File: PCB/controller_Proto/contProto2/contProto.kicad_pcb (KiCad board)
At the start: 2 copper layers, 130.9 x 105.1 mm, 84 parts, among them J1 JST_1mm_4, J10 JST_1mm_3, J11 JST_1mm_3, J12 Conn_01x03_Socket, J13 Conn_01x02_Socket, J14 Conn_01x02_Socket, J15 Conn_01x04, J16 Conn_01x04, J17 Conn_01x10_Pin, J18 JST_1mm_3, J19 Conn_01x08_Socket, J2 Conn_01x04, J20 JST_1mm_4, J22 JST_1mm_4, J23 Conn_01x03_Socket, J24 Conn_01x03_Socket, J25 Conn_01x03_Socket, J26 Conn_01x03_Socket, J27 Conn_01x03_Socket, J28 Conn_01x12_Socket, J29 Conn_01x12_Socket, J3 Conn_01x10_Pin, J30 Conn_01x12_Socket, J31 Conn_01x12_Socket, J32 Conn_01x03_Socket, J33 Conn_01x03_Socket, J36 Conn_01x05, J37 Conn_01x05, J4 JST_1mm_3, J5 Conn_01x02_Socket, J6 JST_1mm_3, J7 Conn_01x02_Socket, J8 JST_1mm_4, J9 Conn_01x04, SW1 SMD_12x12mm_h8.5mm, SW10 SMD_12x12mm_h8.5mm, SW11 SMD_12x12mm_h8.5mm, SW12 SMD_12x12mm_h8.5mm, SW13 SMD_12x12mm_h8.5mm, SW14 SMD_12x12mm_h8.5mm, SW15 SMD_12x12mm_h8.5mm, SW16 SMD_12x12mm_h8.5mm, SW17 SMD_12x12mm_h8.5mm, SW18 SMD_12x12mm_h8.5mm, SW19 SMD_12x12mm_h8.5mm, SW2 SMD_12x12mm_h8.5mm, SW20 SMD_12x12mm_h8.5mm, SW3 SMD_12x12mm_h8.5mm, SW4 SMD_12x12mm_h8.5mm, SW5 SMD_12x12mm_h8.5mm, SW6 SMD_12x12mm_h8.5mm, SW7 SMD_12x12mm_h8.5mm, SW8 SMD_12x12mm_h8.5mm, SW9 SMD_12x12mm_h8.5mm, U1 ProMicroC, U2 ProMicroC, U3 DRV5033FAxLPG, U4 DRV5033FAxLPG

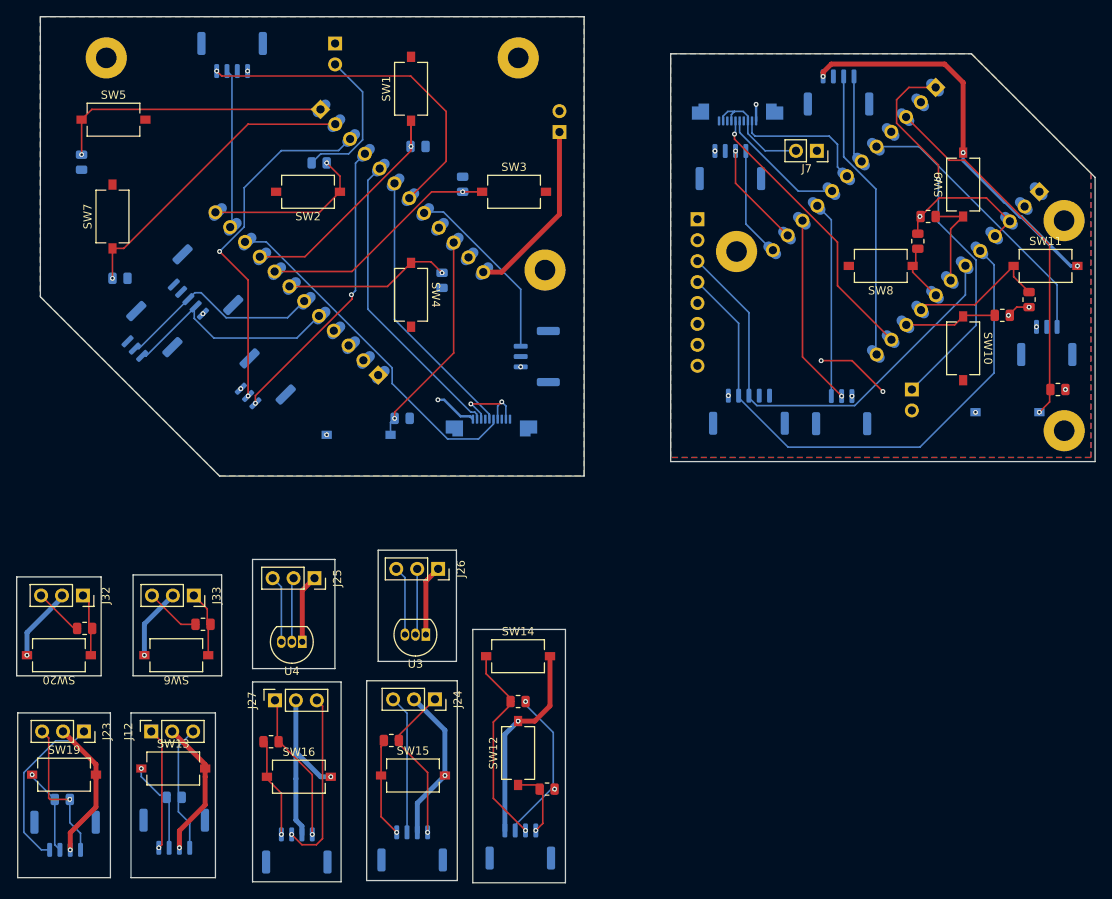
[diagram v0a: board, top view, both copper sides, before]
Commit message: final pcb
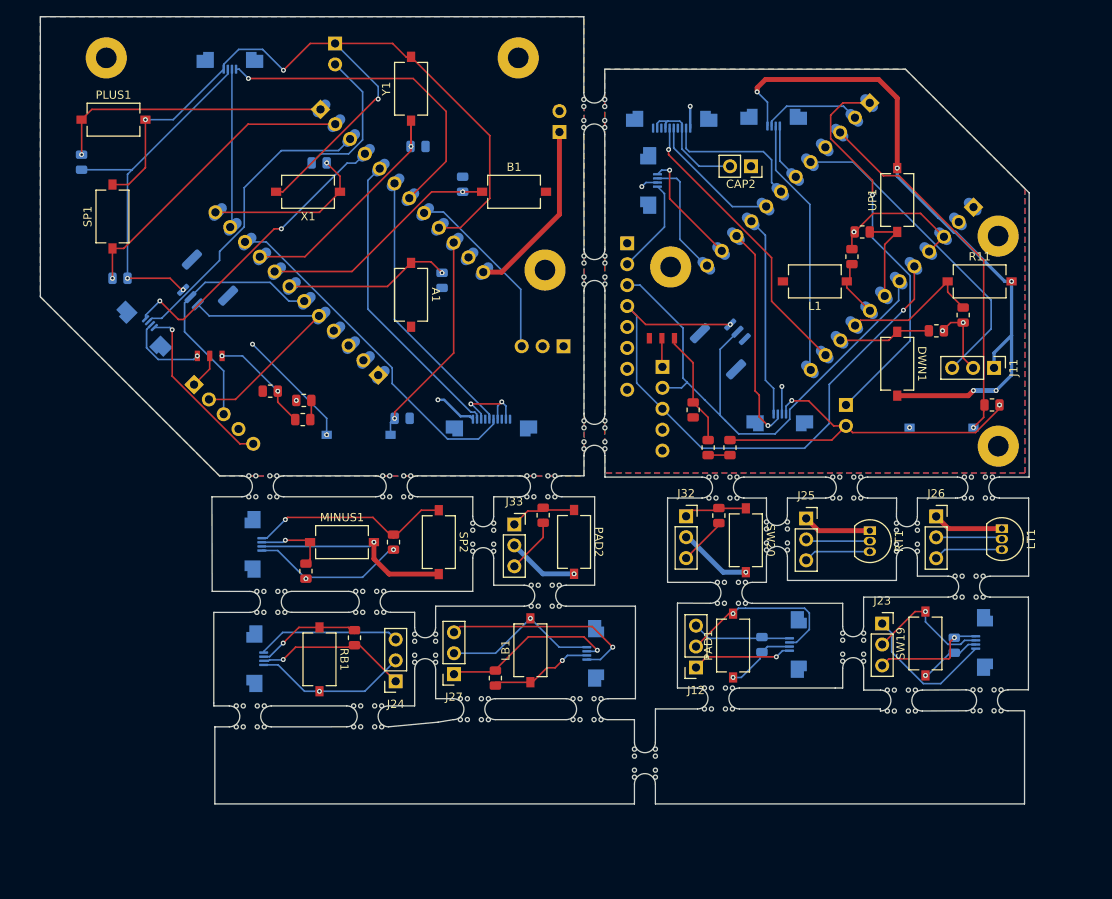
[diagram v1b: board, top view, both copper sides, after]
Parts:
- removed J1, J20, J22, J8: JST_1mm_4, Connector_JST:JST_GH_BM04B-GHS-TBT_1x04-1MP_P1.25mm_Vertical
- removed J15, J16, J2: Conn_01x04, Connector_JST:JST_GH_BM04B-GHS-TBT_1x04-1MP_P1.25mm_Vertical
- removed J36: Conn_01x05, Connector_JST:JST_GH_BM05B-GHS-TBT_1x05-1MP_P1.25mm_Vertical
- removed J6: JST_1mm_3, Connector_JST:JST_GH_BM03B-GHS-TBT_1x03-1MP_P1.25mm_Vertical
- added JP1: ~, PCM_SparkFun-Jumper:Jumper_3_NO, F.Cu at (99.9, 61.5)
- added JP2: ~, PCM_SparkFun-Jumper:Jumper_3_NO, F.Cu at (45.0, 63.7)
- added L_SHOUL1: Conn_01x04, Connector_FFC-FPC:Amphenol_F32Q-1A7x1-11004_1x04-1MP_P0.5mm_Horizontal, B.Cu at (93.7, 99.8)
- added PAD3: Conn_01x04, Connector_FFC-FPC:Amphenol_F32Q-1A7x1-11004_1x04-1MP_P0.5mm_Horizontal, B.Cu at (35.8, 61.8)
- added PAD4: Conn_01x04, Connector_FFC-FPC:Amphenol_F32Q-1A7x1-11004_1x04-1MP_P0.5mm_Horizontal, B.Cu at (114.2, 73.6)
- added PAD_B1: Conn_01x04, Connector_FFC-FPC:Amphenol_F32Q-1A7x1-11004_1x04-1MP_P0.5mm_Horizontal, B.Cu at (118.3, 98.7)
- added PAD_B2: Conn_01x04, Connector_FFC-FPC:Amphenol_F32Q-1A7x1-11004_1x04-1MP_P0.5mm_Horizontal, B.Cu at (140.9, 98.5)
- added R12: 1k, PCM_SparkFun-Resistor:R_0805_2012Metric, F.Cu at (52.4, 68.0)
- added R23: 1k, PCM_SparkFun-Resistor:R_0805_2012Metric, F.Cu at (56.4, 71.4)
- added R24: 1k, PCM_SparkFun-Resistor:R_0805_2012Metric, F.Cu at (103.7, 70.2)
- added R25: 1k, PCM_SparkFun-Resistor:R_0805_2012Metric, F.Cu at (105.5, 74.8)
- added R26: 1k, PCM_SparkFun-Resistor:R_0805_2012Metric, F.Cu at (56.5, 69.1)
- added R27: 1k, PCM_SparkFun-Resistor:R_0805_2012Metric, F.Cu at (108.2, 74.8)
- added REF**: MouseBite-Slot_2.54x2.54mm_on-edge_D0.5mm_P0.85mm_4h_Trace, Panelization:MouseBite-Slot_2.54x2.54mm_on-edge_D0.5mm_P0.85mm_4h_Trace, F.Cu at (52.5, 92.3)
- added REF**: MouseBite-Slot_2.54x2.54mm_on-edge_D0.5mm_P0.85mm_4h_Trace, Panelization:MouseBite-Slot_2.54x2.54mm_on-edge_D0.5mm_P0.85mm_4h_Trace, F.Cu at (64.5, 92.2)
- added REF**: MouseBite-Slot_2.54x2.54mm_on-edge_D0.5mm_P0.85mm_4h_Trace, Panelization:MouseBite-Slot_2.54x2.54mm_on-edge_D0.5mm_P0.85mm_4h_Trace, F.Cu at (137.2, 90.4)
- added REF**: MouseBite-Slot_2.54x2.54mm_on-edge_D0.5mm_P0.85mm_4h_Trace, Panelization:MouseBite-Slot_2.54x2.54mm_on-edge_D0.5mm_P0.85mm_4h_Trace, F.Cu at (122.4, 78.4)
- added REF**: MouseBite-Slot_2.54x2.54mm_on-edge_D0.5mm_P0.85mm_4h_Trace, Panelization:MouseBite-Slot_2.54x2.54mm_on-edge_D0.5mm_P0.85mm_4h_Trace, F.Cu at (124.4, 99.0)
- added REF**: MouseBite-Slot_2.54x2.54mm_on-edge_D0.5mm_P0.85mm_4h_Trace, Panelization:MouseBite-Slot_2.54x2.54mm_on-edge_D0.5mm_P0.85mm_4h_Trace, F.Cu at (50.0, 106.2)
- added REF**: MouseBite-Slot_2.54x2.54mm_on-edge_D0.5mm_P0.85mm_4h_Trace, Panelization:MouseBite-Slot_2.54x2.54mm_on-edge_D0.5mm_P0.85mm_4h_Trace, F.Cu at (106.8, 104.0)
- added REF**: MouseBite-Slot_2.54x2.54mm_on-edge_D0.5mm_P0.85mm_4h_Trace, Panelization:MouseBite-Slot_2.54x2.54mm_on-edge_D0.5mm_P0.85mm_4h_Trace, F.Cu at (93.0, 34.2)
- added REF**: MouseBite-Slot_2.54x2.54mm_on-edge_D0.5mm_P0.85mm_4h_Trace, Panelization:MouseBite-Slot_2.54x2.54mm_on-edge_D0.5mm_P0.85mm_4h_Trace, F.Cu at (93.0, 53.2)
- added REF**: MouseBite-Slot_2.54x2.54mm_on-edge_D0.5mm_P0.85mm_4h_Trace, Panelization:MouseBite-Slot_2.54x2.54mm_on-edge_D0.5mm_P0.85mm_4h_Trace, F.Cu at (129.0, 104.2)
- added REF**: MouseBite-Slot_2.54x2.54mm_on-edge_D0.5mm_P0.85mm_4h_Trace, Panelization:MouseBite-Slot_2.54x2.54mm_on-edge_D0.5mm_P0.85mm_4h_Trace, F.Cu at (79.5, 85.7)
- added REF**: MouseBite-Slot_2.54x2.54mm_on-edge_D0.5mm_P0.85mm_4h_Trace, Panelization:MouseBite-Slot_2.54x2.54mm_on-edge_D0.5mm_P0.85mm_4h_Trace, F.Cu at (67.8, 78.2)
- added REF**: MouseBite-Slot_2.54x2.54mm_on-edge_D0.5mm_P0.85mm_4h_Trace, Panelization:MouseBite-Slot_2.54x2.54mm_on-edge_D0.5mm_P0.85mm_4h_Trace, F.Cu at (77.2, 105.3)
- added REF**: MouseBite-Slot_2.54x2.54mm_on-edge_D0.5mm_P0.85mm_4h_Trace, Panelization:MouseBite-Slot_2.54x2.54mm_on-edge_D0.5mm_P0.85mm_4h_Trace, F.Cu at (51.5, 78.2)
- added REF**: MouseBite-Slot_2.54x2.54mm_on-edge_D0.5mm_P0.85mm_4h_Trace, Panelization:MouseBite-Slot_2.54x2.54mm_on-edge_D0.5mm_P0.85mm_4h_Trace, F.Cu at (90.8, 105.3)
- added REF**: MouseBite-Slot_2.54x2.54mm_on-edge_D0.5mm_P0.85mm_4h_Trace, Panelization:MouseBite-Slot_2.54x2.54mm_on-edge_D0.5mm_P0.85mm_4h_Trace, F.Cu at (112.6, 85.5)
- added REF**: MouseBite-Slot_2.54x2.54mm_on-edge_D0.5mm_P0.85mm_4h_Trace, Panelization:MouseBite-Slot_2.54x2.54mm_on-edge_D0.5mm_P0.85mm_4h_Trace, F.Cu at (93.0, 73.2)
- added REF**: MouseBite-Slot_2.54x2.54mm_on-edge_D0.5mm_P0.85mm_4h_Trace, Panelization:MouseBite-Slot_2.54x2.54mm_on-edge_D0.5mm_P0.85mm_4h_Trace, F.Cu at (138.3, 78.4)
- added REF**: MouseBite-Slot_2.54x2.54mm_on-edge_D0.5mm_P0.85mm_4h_Trace, Panelization:MouseBite-Slot_2.54x2.54mm_on-edge_D0.5mm_P0.85mm_4h_Trace, F.Cu at (139.4, 106.7)
- added REF**: MouseBite-Slot_2.54x2.54mm_on-edge_D0.5mm_P0.85mm_4h_Trace, Panelization:MouseBite-Slot_2.54x2.54mm_on-edge_D0.5mm_P0.85mm_4h_Trace, F.Cu at (85.8, 91.5)
- added REF**: MouseBite-Slot_2.54x2.54mm_on-edge_D0.5mm_P0.85mm_4h_Trace, Panelization:MouseBite-Slot_2.54x2.54mm_on-edge_D0.5mm_P0.85mm_4h_Trace, F.Cu at (85.2, 78.2)
- added REF**: MouseBite-Slot_2.54x2.54mm_on-edge_D0.5mm_P0.85mm_4h_Trace, Panelization:MouseBite-Slot_2.54x2.54mm_on-edge_D0.5mm_P0.85mm_4h_Trace, F.Cu at (108.4, 91.2)
- added REF**: MouseBite-Slot_2.54x2.54mm_on-edge_D0.5mm_P0.85mm_4h_Trace, Panelization:MouseBite-Slot_2.54x2.54mm_on-edge_D0.5mm_P0.85mm_4h_Trace, F.Cu at (99.1, 113.1)
- added REF**: MouseBite-Slot_2.54x2.54mm_on-edge_D0.5mm_P0.85mm_4h_Trace, Panelization:MouseBite-Slot_2.54x2.54mm_on-edge_D0.5mm_P0.85mm_4h_Trace, F.Cu at (72.5, 99.2)
- added REF**: MouseBite-Slot_2.54x2.54mm_on-edge_D0.5mm_P0.85mm_4h_Trace, Panelization:MouseBite-Slot_2.54x2.54mm_on-edge_D0.5mm_P0.85mm_4h_Trace, F.Cu at (107.3, 78.4)
- added REF**: MouseBite-Slot_2.54x2.54mm_on-edge_D0.5mm_P0.85mm_4h_Trace, Panelization:MouseBite-Slot_2.54x2.54mm_on-edge_D0.5mm_P0.85mm_4h_Trace, F.Cu at (130.9, 85.7)
- added REF**: MouseBite-Slot_2.54x2.54mm_on-edge_D0.5mm_P0.85mm_4h_Trace, Panelization:MouseBite-Slot_2.54x2.54mm_on-edge_D0.5mm_P0.85mm_4h_Trace, F.Cu at (64.2, 106.2)
- added R_SHOUL1: Conn_01x04, Connector_FFC-FPC:Amphenol_F32Q-1A7x1-11004_1x04-1MP_P0.5mm_Horizontal, B.Cu at (48.7, 100.4)
- added R_SHOULD1: Conn_01x04, Connector_FFC-FPC:Amphenol_F32Q-1A7x1-11004_1x04-1MP_P0.5mm_Horizontal, B.Cu at (47.5, 26.0)
- added SP_L1: Conn_01x04, Connector_FFC-FPC:Amphenol_F32Q-1A7x1-11004_1x04-1MP_P0.5mm_Horizontal, B.Cu at (96.5, 42.4)
- added SP_LB1: Conn_01x04, Connector_FFC-FPC:Amphenol_F32Q-1A7x1-11004_1x04-1MP_P0.5mm_Horizontal, B.Cu at (48.5, 86.5)
- added TRACK_B1: Conn_01x05, Connector_PinHeader_2.54mm:PinHeader_1x05_P2.54mm_Vertical, B.Cu at (100.0, 65.0)
- J11: footprint Connector_JST:JST_GH_BM03B-GHS-TBT_1x03-1MP_P1.25mm_Vertical -> Connector_PinHeader_2.54mm:PinHeader_1x03_P2.54mm_Vertical; moved to F.Cu
- J9: footprint Connector_JST:JST_GH_BM04B-GHS-TBT_1x04-1MP_P1.25mm_Vertical -> Connector_FFC-FPC:Amphenol_F32Q-1A7x1-11004_1x04-1MP_P0.5mm_Horizontal
- RUMBLE1: renamed from J10; footprint Connector_JST:JST_GH_BM03B-GHS-TBT_1x03-1MP_P1.25mm_Vertical -> Connector_PinHeader_2.54mm:PinHeader_1x03_P2.54mm_Vertical
- TRACK_B2: renamed from J37; value Conn_01x05 -> TRACK_B; footprint Connector_JST:JST_GH_BM05B-GHS-TBT_1x05-1MP_P1.25mm_Vertical -> Connector_PinHeader_2.54mm:PinHeader_1x05_P2.54mm_Vertical
- moved R4 109.9 mm to (135.4, 98.8), turned to 90 degrees
- moved SW19 105.8 mm to (131.9, 98.6), turned to 90 degrees
- moved J23 97.8 mm to (126.7, 96.2), turned to 0 degrees
- moved SW20 84.5 mm to (110.1, 86.0), turned to -90 degrees
- moved R1 78.2 mm to (106.8, 83.0), turned to -90 degrees
- moved J32 73.8 mm to (102.9, 83.1), turned to 0 degrees
- moved R17 73.7 mm to (112.1, 98.7), turned to 90 degrees
- moved LT1 71.1 mm to (141.2, 84.6), turned to -90 degrees
- moved RT1 70.2 mm to (125.2, 84.9), turned to -90 degrees
- moved PAD1 69.6 mm to (108.6, 98.8), turned to 90 degrees
- moved J12 66.6 mm to (104.1, 101.5), turned to 180 degrees
- moved J26 60.8 mm to (133.2, 83.2), turned to 0 degrees
- moved J25 60.1 mm to (117.5, 83.4), turned to 0 degrees
- moved J18 56.9 mm to (107.7, 62.1), turned to -45 degrees
- moved PAD2 50.2 mm to (89.3, 86.2), turned to -90 degrees
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- renumbered SW4 to A1, SW3 to B1, J5 to CAP1, J7 to CAP2, SW10 to DWN1, J4 to I2C1, J3 to JOY_R1, SW8 to L1, SW16 to LB1, U3 to LT1, SW12 to MINUS1, J19 to MPU1, SW13 to PAD1, SW6 to PAD2, SW5 to PLUS1, SW11 to R11, SW15 to RB1, SW17 to RST1, SW18 to RST2, U4 to RT1, SW7 to SP1, SW14 to SP2, SW9 to UP1, J14 to VIN1, J13 to VIN2, SW2 to X1, SW1 to Y1
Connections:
- J18 pad 1: /Pad2 -> SDA2
- J18 pad 2: /Pad1 -> SCL2
- J18 pad 3: VCC -> GND2
- TRACK_B2 pad 1: VCC -> /TB_in2
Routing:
- net VCC: track 5.22 -> 134.5 mm, vias 6 -> 7
- net GND2: track 43.9 -> 110.1 mm, vias 6 -> 5
- net GND: track 28.8 -> 94.6 mm, vias 2 -> 6
- net VCC2: track 49.5 -> 91.4 mm
- net 3.3v2: track 0.00 -> 14.1 mm
- net SCL2: track 54.9 -> 68.5 mm
- net 3.3V1: track 0.00 -> 12.9 mm, vias 0 -> 2
- net SCL: track 25.5 -> 32.0 mm
- net /Pad1: track 43.3 -> 37.1 mm, vias 2 -> 0
- net SDA2: track 68.8 -> 74.8 mm, vias 0 -> 2
- net SDA: track 27.7 -> 32.9 mm
- net /A32: track 34.0 -> 39.0 mm
- net /TB_in2: track 0.00 -> 4.27 mm
- net /L1: track 35.3 -> 31.3 mm
- net /PPVCC1: track 17.1 -> 21.0 mm
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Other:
- board size 130.9 x 105.1 mm -> 120 x 95.5 mm
